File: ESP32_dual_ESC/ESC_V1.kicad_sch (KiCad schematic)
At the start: 40 parts, among them J1 A, J2 B, J3 C, Q1 HYG025N06LS1C2, Q2 HYG025N06LS1C2, Q3 HYG025N06LS1C2, Q4 HYG025N06LS1C2, Q5 HYG025N06LS1C2, Q6 HYG025N06LS1C2, U1 LM324, U2 LM5109BMA, U3 LM5109BMA, U4 LM5109BMA

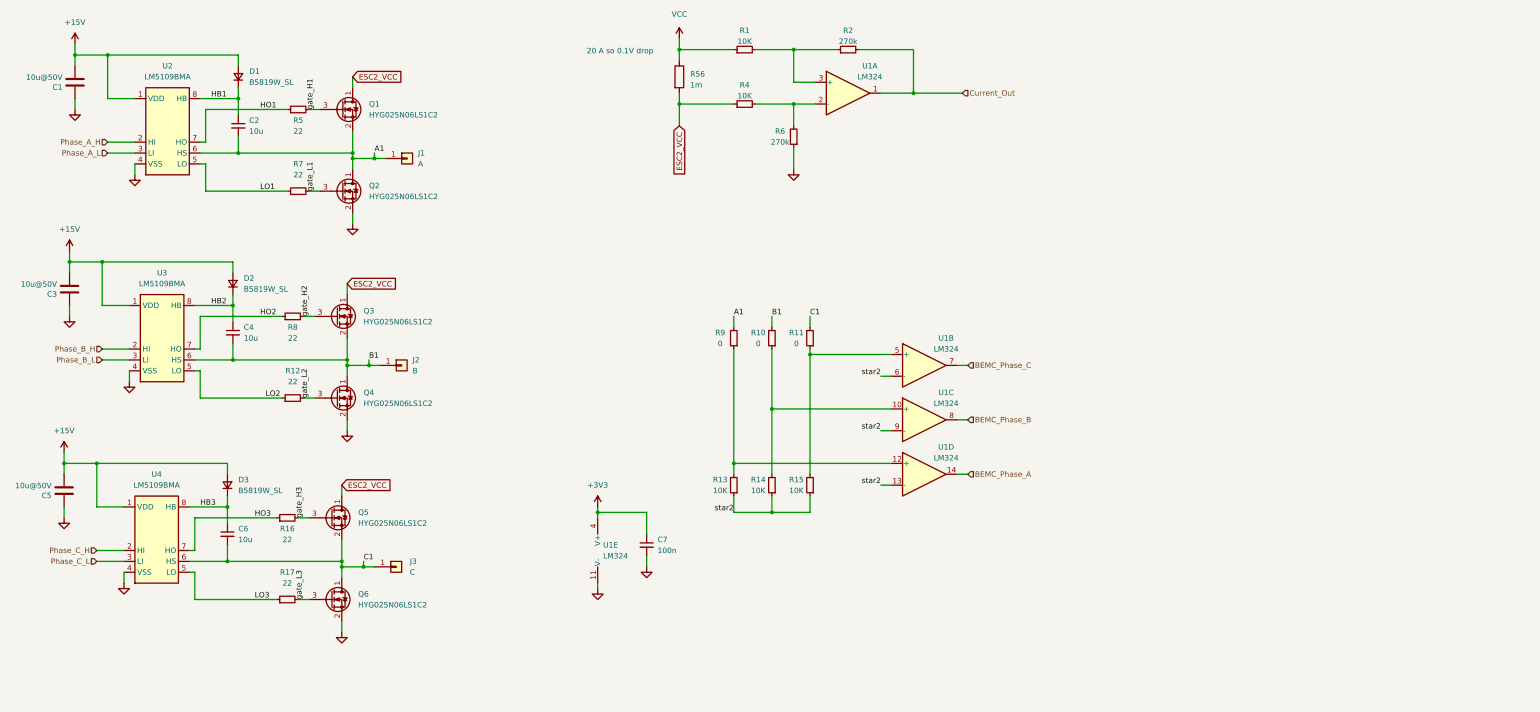
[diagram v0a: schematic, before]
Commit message: g
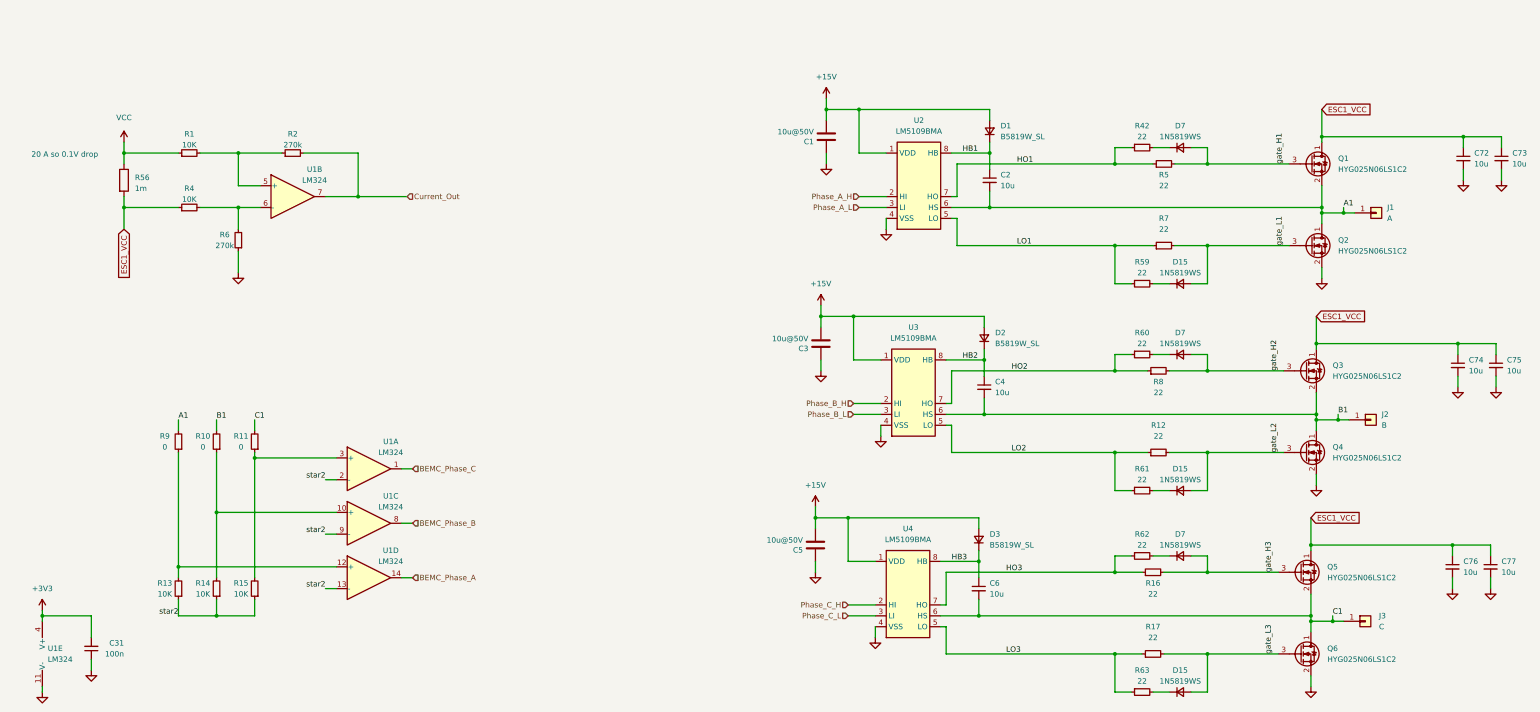
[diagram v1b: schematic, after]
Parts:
- removed C7: 100n, symbol Device:C_Small
- added C31: 100n, Capacitor_SMD:C_0603_1608Metric, symbol Device:C_Small
- added C72, C73, C74, C75, C76, C77: 10u, Capacitor_SMD:C_1206_3216Metric, symbol Device:C_Small
- added D15 (x3), D7 (x3): 1N5819WS, Diode_SMD:D_SOD-323, symbol Device:D_Small
- added R42, R59, R60, R61, R62, R63: 22, Resistor_SMD:R_0603_1608Metric, symbol Device:R_Small
- C2, C4, C6: footprint Capacitor_SMD:C_0603_1608Metric -> Capacitor_SMD:C_0805_2012Metric; LCSC C96446 -> C15850
- J1, J2, J3: footprint Mounting_Wuerth:Mounting_Wuerth_WA-SMSI-M1.6_H1.5mm_9774015633 -> MountingHole:MountingHole_2.5mm_Pad_TopBottom
- R1, R4: footprint (none) -> Resistor_SMD:R_0603_1608Metric; LCSC (none) -> C25804
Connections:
- net +3V3: now also C31.2
- net BEMC_Phase_C: now also U1.1; no longer U1.7
- net Current_Out: now also U1.7; no longer U1.1
- net GND: now also C31.1, C72.2, C73.2, C74.2, C75.2, C76.2, C77.2
- net HO1: now also R42.1
- net HO2: now also R60.1
- net HO3: now also R62.1
- net LO1: now also R59.1
- net LO2: now also R61.1
- net LO3: now also R63.1
- net gate_H1: now also D7.2 (A)
- net gate_H2: now also D7.2 (A)
- net gate_H3: now also D7.2 (A)
- net gate_L1: now also D15.2 (A)
- net gate_L2: now also D15.2 (A)
- net gate_L3: now also D15.2 (A)
- net star2: now also U1.2 (-); no longer U1.6 (-)
- net at R4.2, R6.2: now also U1.6 (-); no longer U1.2 (-)
- net at R11.1, R15.2: now also U1.3 (+); no longer U1.5 (+)
- net at R1.2, R2.1: now also U1.5 (+); no longer U1.3 (+)
- net ESC2_VCC renamed ESC1_VCC
- net ESC1_VCC: now also C72.1, C73.1, C74.1, C75.1, C76.1, C77.1
- new net: D7.1 (K), R42.2
- new net: D15.1 (K), R63.2
- new net: D15.1 (K), R61.2
- new net: D15.1 (K), R59.2
- new net: D7.1 (K), R62.2
- new net: D7.1 (K), R60.2
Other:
- moved on the sheet: C1, C3, C5, D1, D2, D3, J1, J2, J3, Q1, Q2, Q3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
